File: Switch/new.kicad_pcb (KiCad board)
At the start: 2 copper layers, 53.5 x 53 mm, 11 parts, among them J1 RJ45, J2 RJ45, J3 RJ45, J4 RJ45, SW1 Driver/Auton, SW2 Enable/Disable, SW3 Pin7, SW4 Pin4, SW5 Pin1

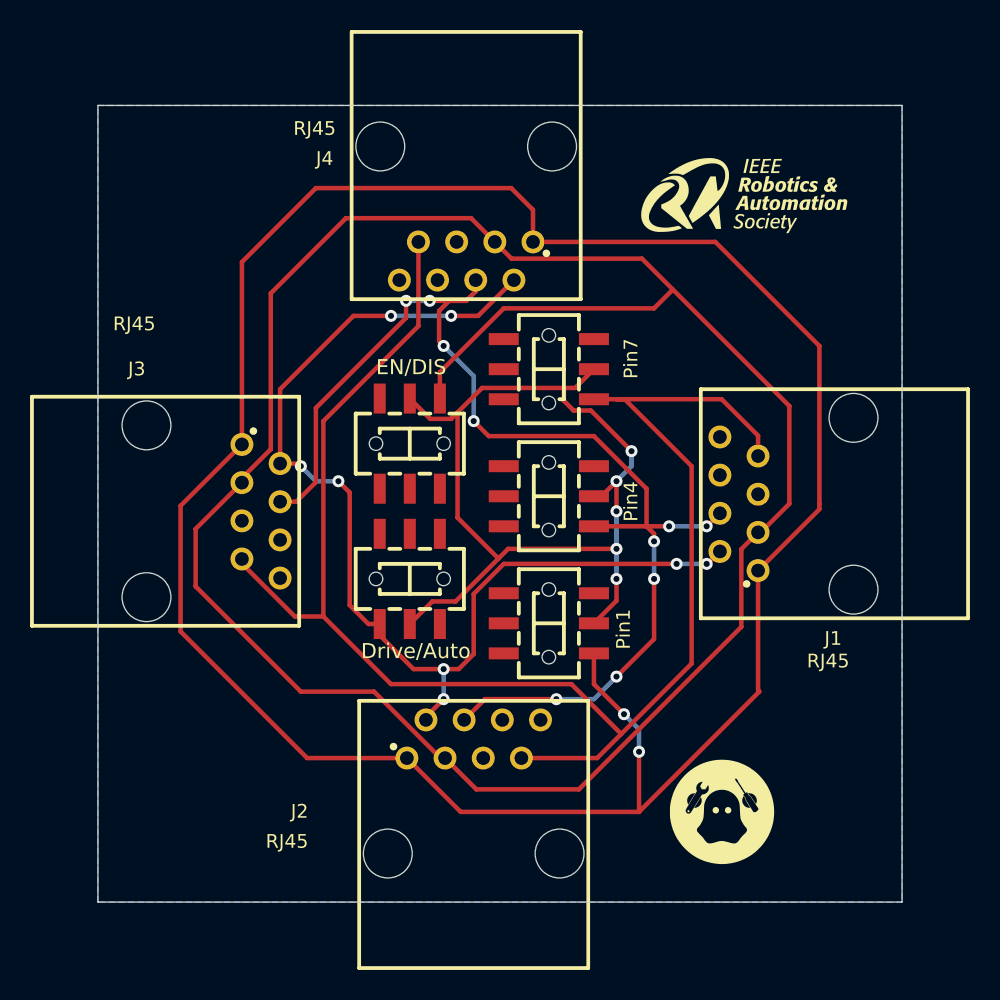
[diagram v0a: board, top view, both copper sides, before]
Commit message: finalize comp switch
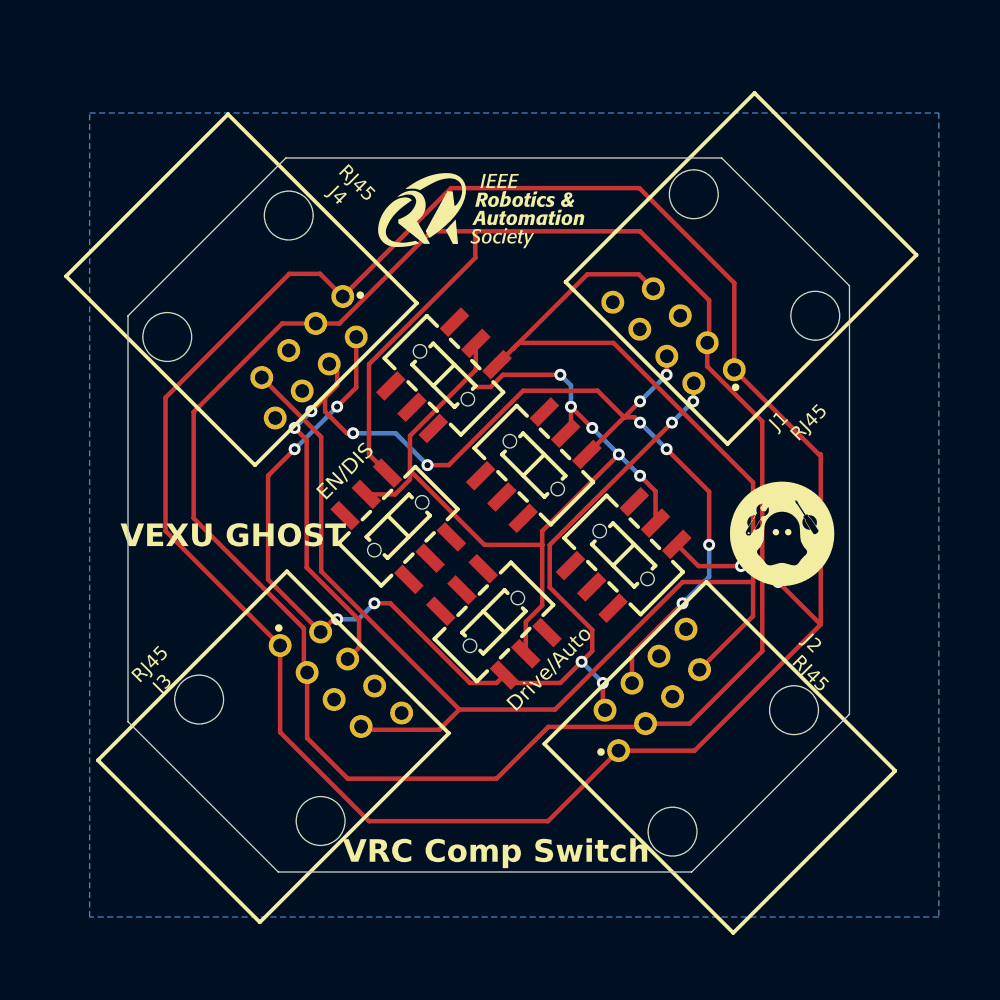
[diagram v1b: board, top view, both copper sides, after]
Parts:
- added G***: LOGO, ghost:ieee, B.Cu at (160.4, 77.4)
- added G***: LOGO, ghost:ghost, B.Cu at (160.5, 93.0)
- J1, J2, J3, J4: footprint RJ45Connector:RJ45-TH_RC0139 -> ghost:RJ45-TH_RC0139
- SW1, SW2, SW3, SW4, SW5: footprint Library:SW-SMD_MS-22D28-G020 -> ghost:SW-SMD_MS-22D28-G020
- moved G*** 18.9 mm to (179.0, 88.0)
- moved G*** 17.5 mm to (159.0, 66.5)
- moved J3 12.4 mm to (149.7, 97.7), turned to 135 degrees
- moved J2 12.3 mm to (170.4, 98.4), turned to -135 degrees
- moved J4 12.3 mm to (147.5, 76.3), turned to 45 degrees
- moved J1 12.0 mm to (171.8, 74.8), turned to -45 degrees
- moved SW3 6.99 mm to (156.5, 77.5), turned to -45 degrees
- moved SW5 6.74 mm to (168.5, 89.4), turned to -45 degrees
- moved SW1 6.28 mm to (159.8, 93.9), turned to -135 degrees
- moved SW2 5.55 mm to (153.5, 87.5), turned to 45 degrees
- moved SW4 2.30 mm to (162.5, 83.4), turned to -45 degrees
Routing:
- net Net-(J1-Pad1): track 155.6 -> 153.7 mm
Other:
- board size 53.5 x 53 mm -> 48 x 47.5 mm
- board text added: "VEXU GHOST"
- board text added: "VRC Comp Switch"
